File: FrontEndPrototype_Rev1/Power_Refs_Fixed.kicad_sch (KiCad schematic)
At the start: 10 parts, among them U10 ADR4530, U4 ADA4807-2ACP, U5 ADP7118-1.8

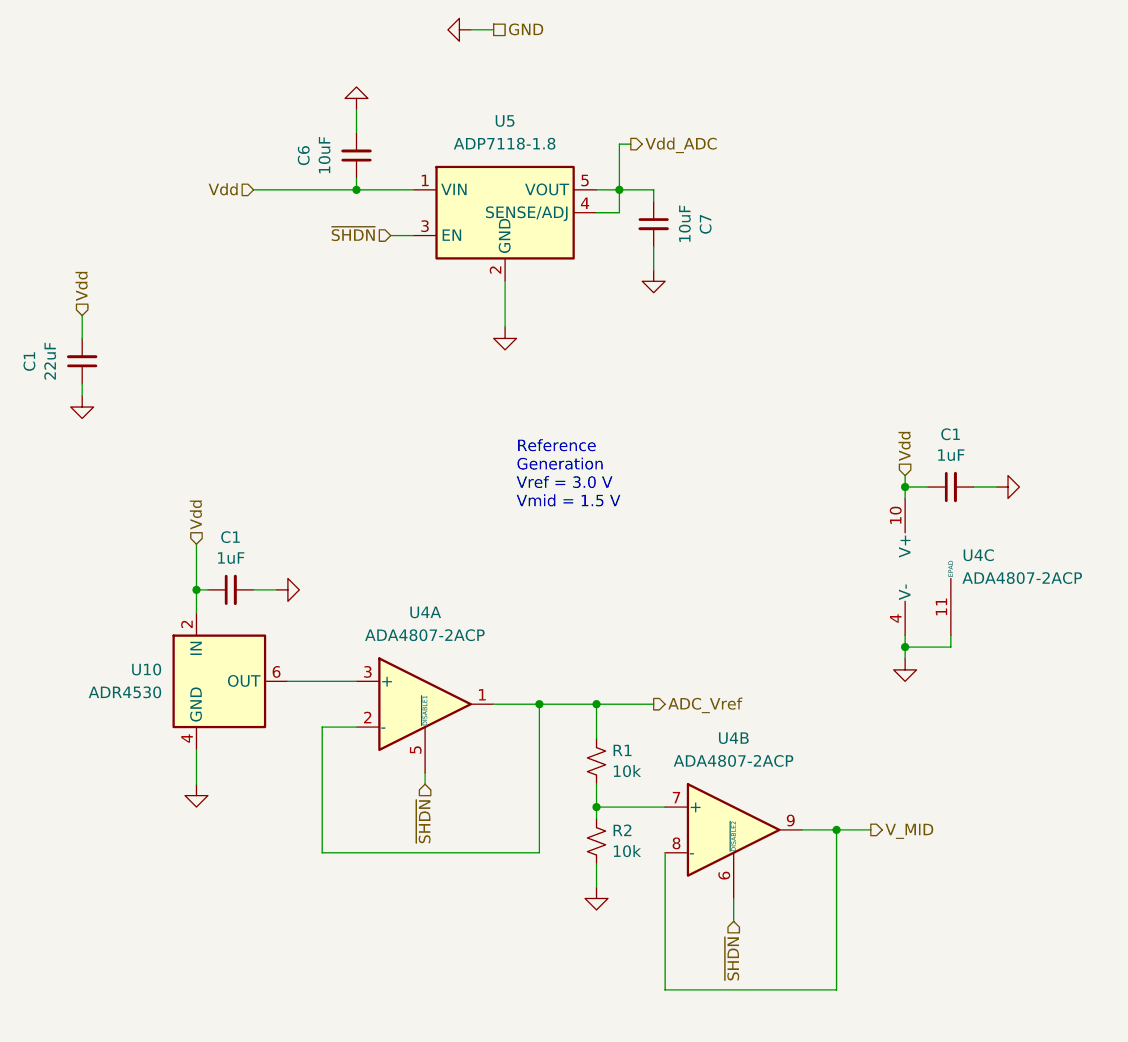
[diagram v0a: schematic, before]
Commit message: Checking if Branch Updates Work
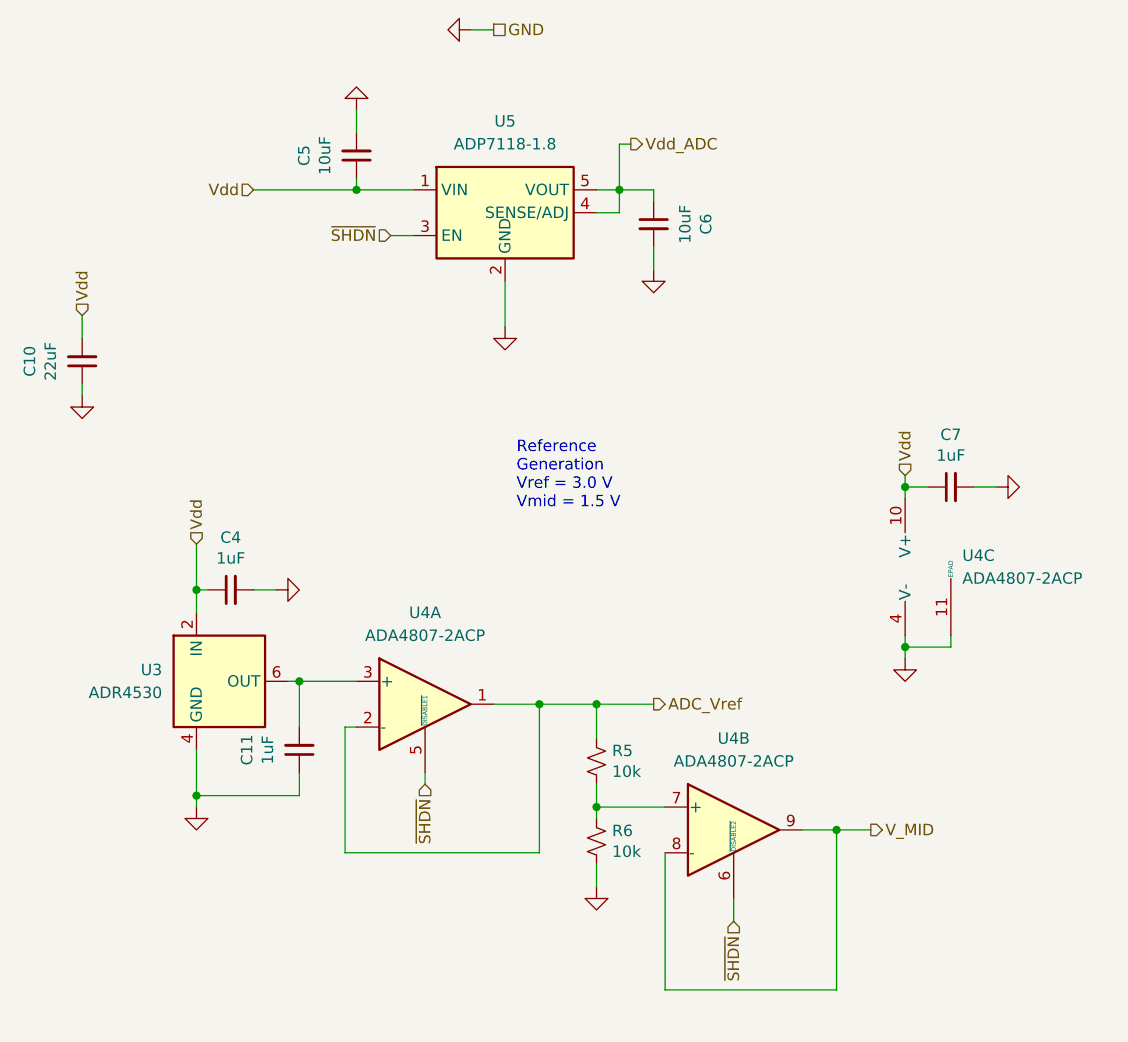
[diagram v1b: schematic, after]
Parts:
- added C11: 1uF, Capacitor_SMD:C_0603_1608Metric_Pad1.08x0.95mm_HandSolder, symbol Device:C_Small
- renumbered C1 to C10, C1 to C4, C6 to C5, C7 to C6, C1 to C7, R1 to R5, R2 to R6, U10 to U3
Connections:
- net GND: now also C11.1
- net at U3.6 (OUT), U4.3 (+): now also C11.2

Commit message: First Pass Schematic Fixes for Power Management Board
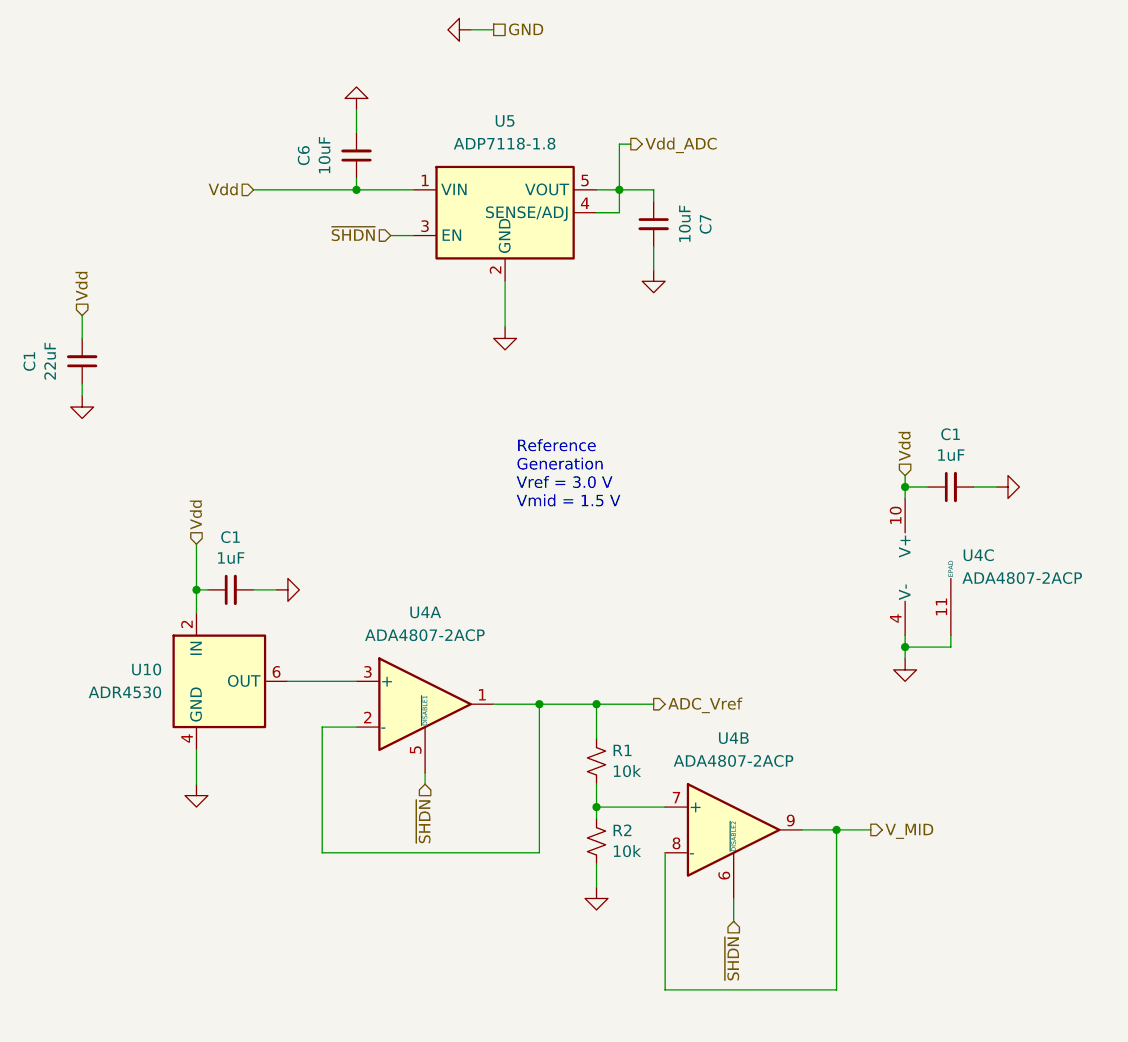
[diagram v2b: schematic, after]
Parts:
- removed C11: 1uF, Capacitor_SMD:C_0603_1608Metric_Pad1.08x0.95mm_HandSolder, symbol Device:C_Small
- renumbered C7 to C1, C10 to C1, C4 to C1, C5 to C6, C6 to C7, R5 to R1, R6 to R2, U3 to U10
